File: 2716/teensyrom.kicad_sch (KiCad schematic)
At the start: 4 parts, among them J1 Conn_01x06_Pin, U1 27512, U2 2716, U3 Teensy 4.1 module

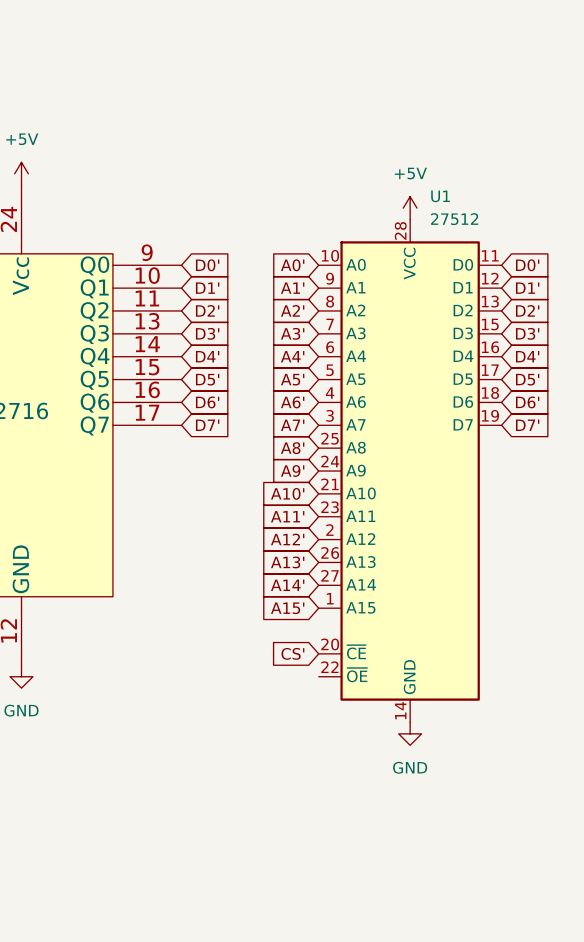
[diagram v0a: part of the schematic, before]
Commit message: update schematic pdfs
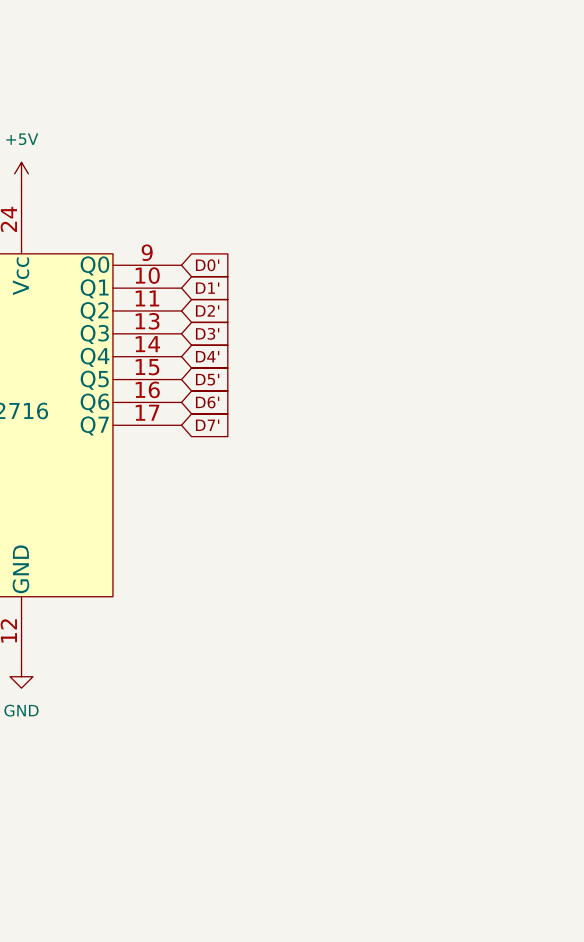
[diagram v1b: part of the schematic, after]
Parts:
- removed U1: 27512, Package_DIP:DIP-28_W15.24mm, symbol Memory_EPROM:27512
